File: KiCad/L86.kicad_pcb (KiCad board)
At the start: 2 copper layers, 38.5 x 30 mm, 4 parts, among them J1 Conn_01x06, U1 L86-M33, U2 QR

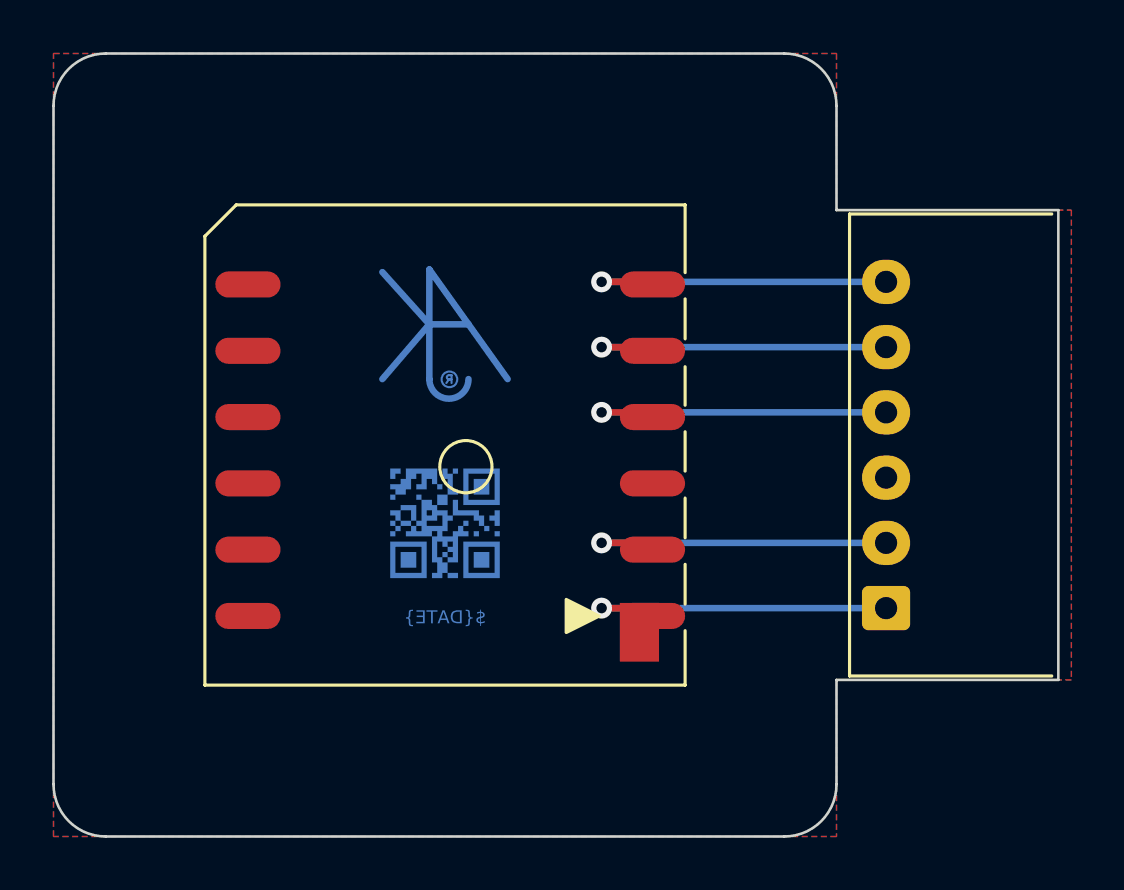
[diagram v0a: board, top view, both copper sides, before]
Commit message: Library update
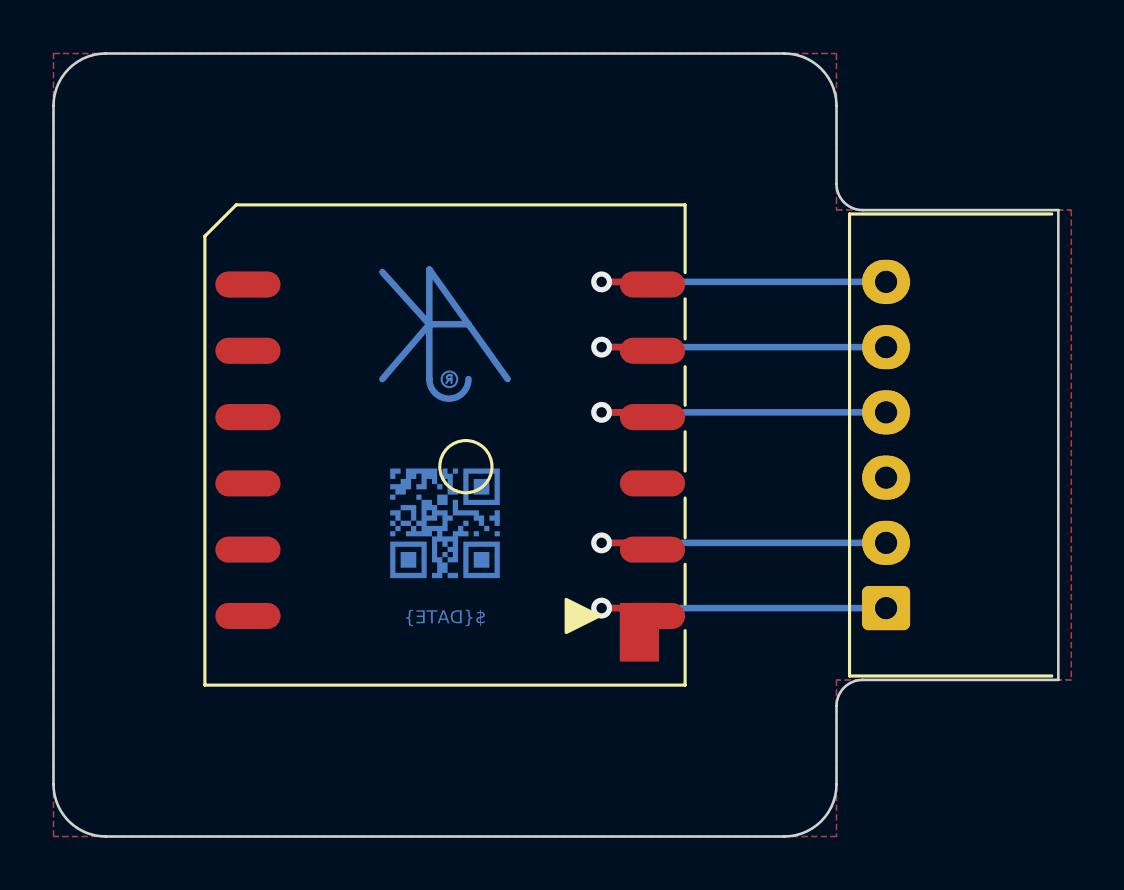
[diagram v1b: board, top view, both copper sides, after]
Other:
- outline, holes or cut-outs redrawn
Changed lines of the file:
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@@
     )
   )
-  (gr_line (start 115 109) (end 115 113) (layer "Edge.Cuts") (width 0.1))
+  (gr_line (start 115 110) (end 115 113) (layer "Edge.Cuts") (width 0.1))
   (gr_arc (start 115 113) (mid 114.414214 114.414214) (end 113 115) (layer "Edge.Cuts") (width 0.1))
   (gr_line (start 87 85) (end 113 85) (layer "Edge.Cuts") (width 0.1))
-  (gr_line (start 115 91) (end 123.5 91) (layer "Edge.Cuts") (width 0.1))
-  (gr_line (start 123.5 109) (end 115 109) (layer "Edge.Cuts") (width 0.1))
+  (gr_line (start 116 91) (end 123.5 91) (layer "Edge.Cuts") (width 0.1))
+  (gr_line (start 123.5 109) (end 116 109) (layer "Edge.Cuts") (width 0.1))
+  (gr_arc (start 116 91) (mid 115.292893 90.707107) (end 115 90) (layer "Edge.Cuts") (width 0.1))
   (gr_arc (start 87 115) (mid 85.585786 114.414214) (end 85 113) (layer "Edge.Cuts") (width 0.1))
+  (gr_arc (start 115 110) (mid 115.292893 109.292893) (end 116 109) (layer "Edge.Cuts") (width 0.1))
   (gr_line (start 113 115) (end 87 115) (layer "Edge.Cuts") (width 0.1))
-  (gr_line (start 115 87) (end 115 91) (layer "Edge.Cuts") (width 0.1))
+  (gr_line (start 115 87) (end 115 90) (layer "Edge.Cuts") (width 0.1))
   (gr_arc (start 113 85) (mid 114.414214 85.585786) (end 115 87) (layer "Edge.Cuts") (width 0.1))
   (gr_arc (start 85 87) (mid 85.585786 85.585786) (end 87 85) (layer "Edge.Cuts") (width 0.1))

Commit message: DRC tweaks
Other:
- rule pad_to_mask_clearance: 0 -> 0.01
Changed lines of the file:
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@@
     (48 "B.Fab" user)
     (49 "F.Fab" user)
-    (50 "User.1" user)
-    (51 "User.2" user)
-    (52 "User.3" user)
-    (53 "User.4" user)
-    (54 "User.5" user)
-    (55 "User.6" user)
-    (56 "User.7" user)
-    (57 "User.8" user)
-    (58 "User.9" user)
   )
   (setup
@@
       (dielectric_constraints no)
     )
-    (pad_to_mask_clearance 0)
+    (pad_to_mask_clearance 0.01)
     (pad_to_paste_clearance_ratio -0.02)
     (pcbplotparams
